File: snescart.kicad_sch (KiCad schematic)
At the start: 6 parts, among them P1 CASSETTE, U3 27C080

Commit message: tracks
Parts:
- C3: footprint Capacitor_THT:C_Disc_D4.3mm_W1.9mm_P5.00mm -> Capacitor_THT:CP_Axial_L10.0mm_D4.5mm_P15.00mm_Horizontal
- U3: footprint (none) -> Package_DIP:DIP-32_W15.24mm
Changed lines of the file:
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@@
       (effects (font (size 1.27 1.27)) (justify left))
     )
-    (property "Footprint" "Capacitor_THT:C_Disc_D4.3mm_W1.9mm_P5.00mm" (at 113.03 23.7998 0)
+    (property "Footprint" "Capacitor_THT:CP_Axial_L10.0mm_D4.5mm_P15.00mm_Horizontal" (at 113.03 23.7998 0)
       (effects (font (size 1.27 1.27)) hide)
     )
@@
       (effects (font (size 1.27 1.27)) (justify right))
     )
-    (property "Footprint" "" (at 69.85 131.445 0)
-      (effects (font (size 1.27 1.27)) hide)
-    )
+    (property "Footprint" "Package_DIP:DIP-32_W15.24mm" (at 69.85 131.445 0)
+      (effects (font (size 1.27 1.27)) hide)
+    )

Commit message: funny cap
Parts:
- C1: footprint Capacitor_THT:C_Disc_D4.3mm_W1.9mm_P5.00mm -> Library:CapacitorSpecial
- C2: footprint Capacitor_THT:C_Disc_D4.3mm_W1.9mm_P5.00mm -> Library:Capacitor
- C3: footprint Capacitor_THT:CP_Axial_L10.0mm_D4.5mm_P15.00mm_Horizontal -> Library:Capacitor
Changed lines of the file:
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@@
       (effects (font (size 1.27 1.27)))
     )
-    (property "Footprint" "Capacitor_THT:C_Disc_D4.3mm_W1.9mm_P5.00mm" (at 48.26 97.4598 0)
+    (property "Footprint" "Library:CapacitorSpecial" (at 48.26 97.4598 0)
       (effects (font (size 1.27 1.27)) hide)
     )
@@
       (effects (font (size 1.27 1.27)) (justify left))
     )
-    (property "Footprint" "Capacitor_THT:CP_Axial_L10.0mm_D4.5mm_P15.00mm_Horizontal" (at 113.03 23.7998 0)
+    (property "Footprint" "Library:Capacitor" (at 113.03 23.7998 0)
       (effects (font (size 1.27 1.27)) hide)
     )
@@
       (effects (font (size 1.27 1.27)) (justify left))
     )
-    (property "Footprint" "Capacitor_THT:C_Disc_D4.3mm_W1.9mm_P5.00mm" (at 150.495 30.7848 0)
+    (property "Footprint" "Library:Capacitor" (at 150.495 30.7848 0)
       (effects (font (size 1.27 1.27)) hide)
     )

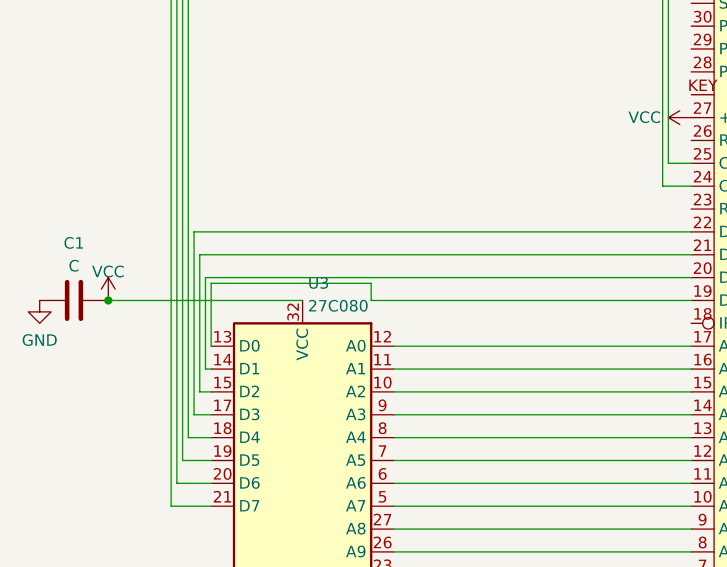
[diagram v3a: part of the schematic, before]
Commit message: date
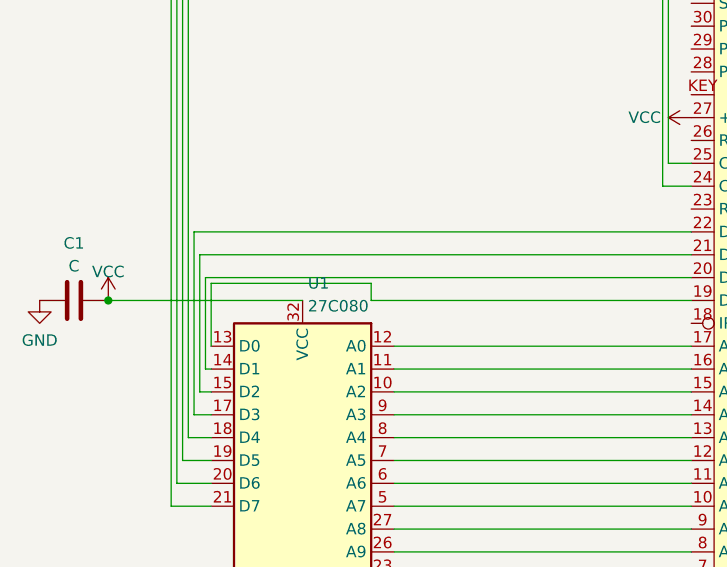
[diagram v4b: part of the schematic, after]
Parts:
- renumbered U3 to U1
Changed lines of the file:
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@@
   (symbol (lib_id "Memory_EPROM:27C080") (at 69.85 131.445 0) (mirror y) (unit 1)
     (in_bom yes) (on_board yes) (dnp no) (fields_autoplaced)
-    (property "Reference" "U3" (at 70.4341 96.52 0)
+    (property "Reference" "U1" (at 70.4341 96.52 0)
       (effects (font (size 1.27 1.27)) (justify right))
     )
@@
       (project "snescart"
         (path "/066a4729-7396-4945-b543-8e17bff58a3f"
-          (reference "U3") (unit 1)
+          (reference "U1") (unit 1)
         )
       )
